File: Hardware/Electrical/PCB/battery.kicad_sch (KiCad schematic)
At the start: 33 parts, among them J2 jst, Q1 DMT6008LFG-7, Q2 DMT6008LFG-7, U6 BQ24600

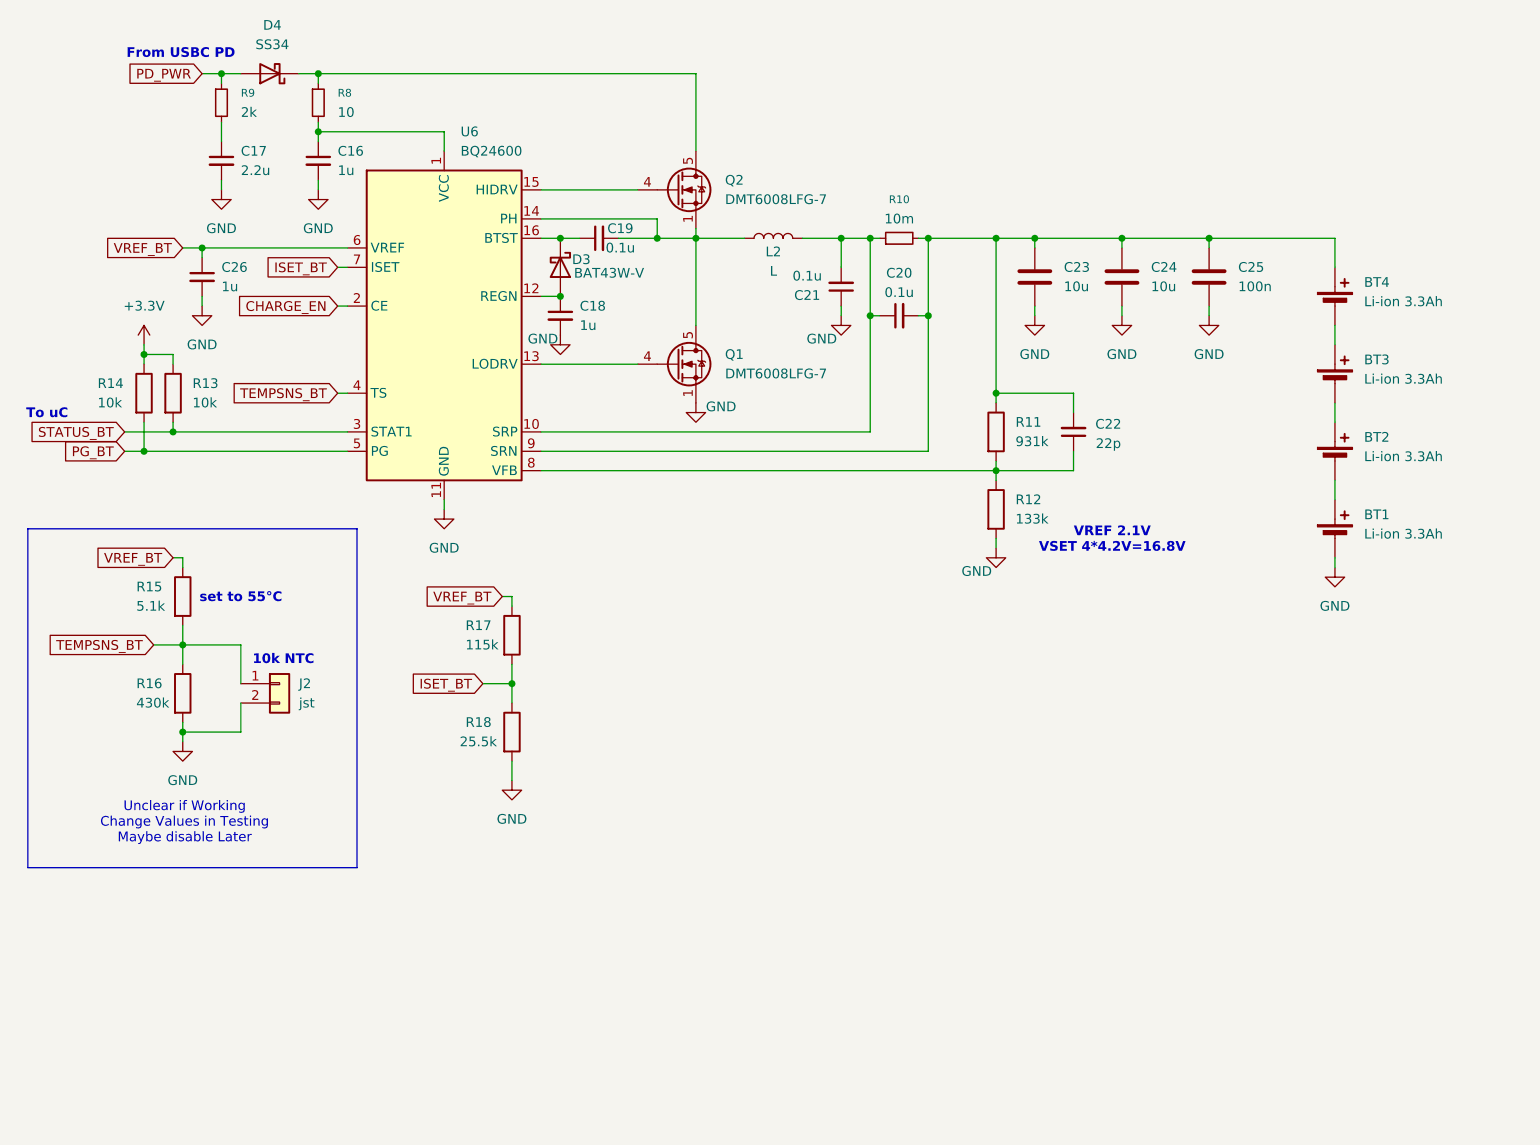
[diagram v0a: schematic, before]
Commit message: project state at start of school project
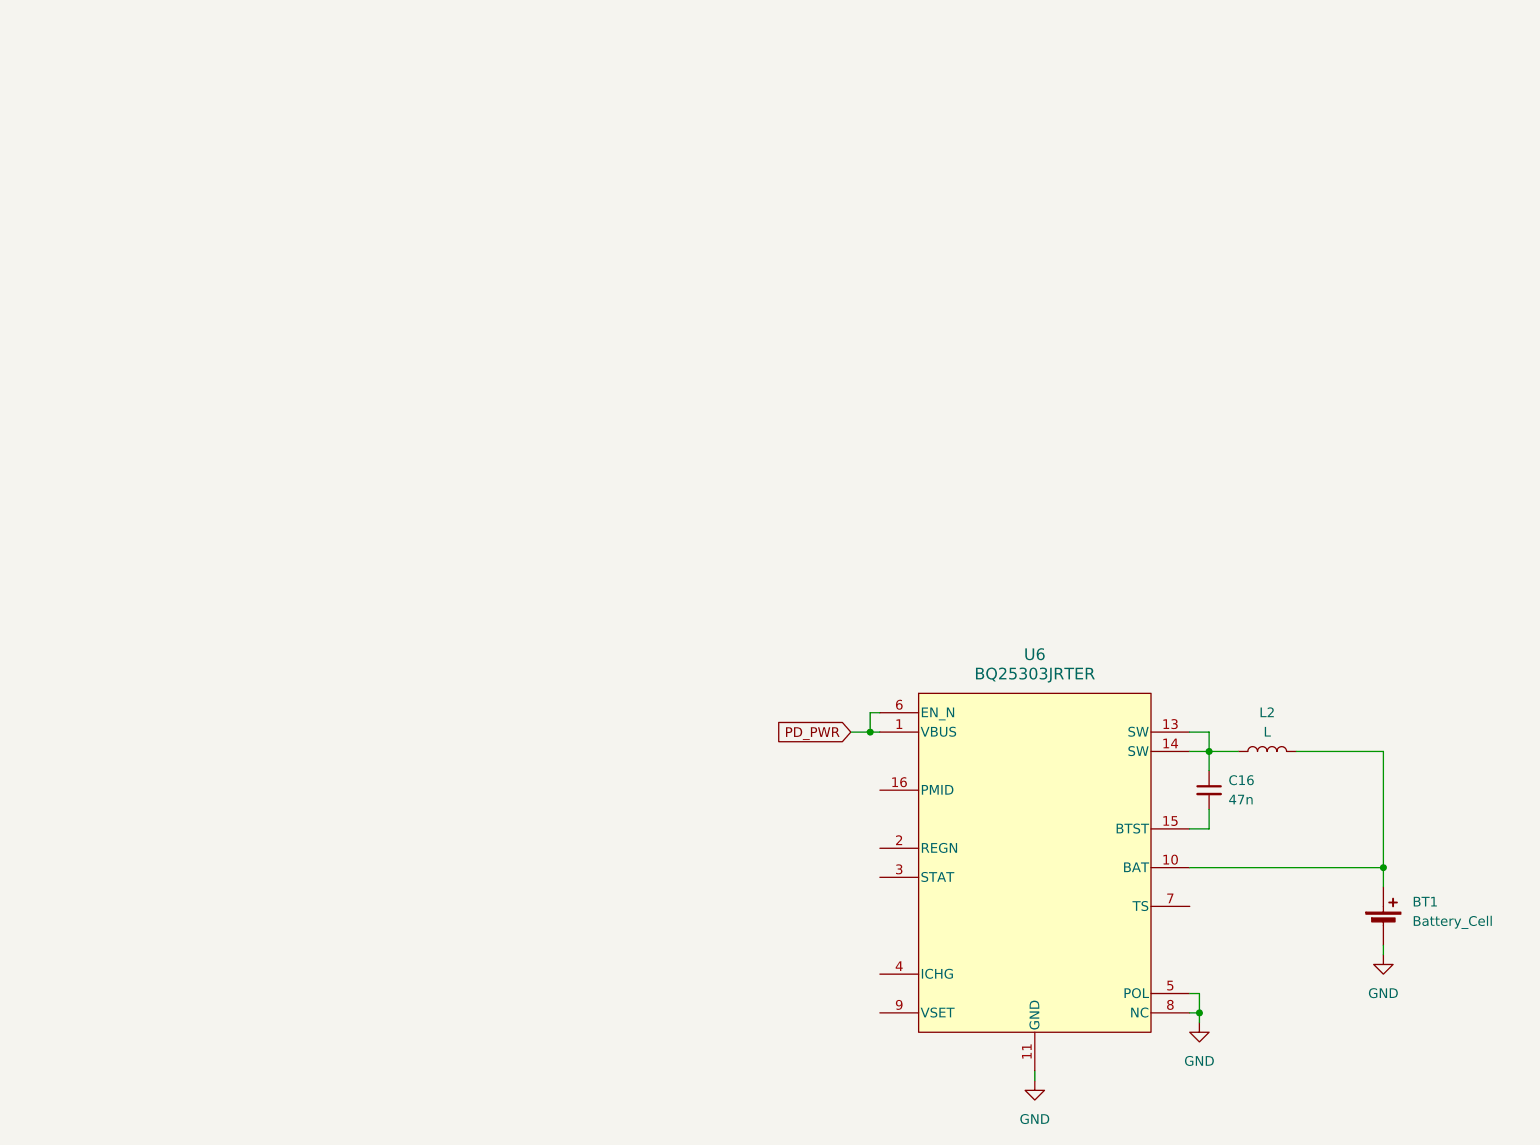
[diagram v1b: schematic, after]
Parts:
- removed BT2, BT3, BT4: Li-ion 3.3Ah, symbol Device:Battery_Cell
- removed C17: 2.2u, symbol Device:C_Small
- removed C18, C26: 1u, symbol Device:C_Small
- removed C19, C20, C21: 0.1u, symbol Device:C_Small
- removed C22: 22p, symbol Device:C_Small
- removed C23, C24: 10u, symbol Device:C
- removed C25: 100n, symbol Device:C
- removed D3: BAT43W-V, Diode_SMD:D_SOD-123, symbol Diode:BAT43W-V
- removed D4: SS34, Diode_SMD:D_SMC, symbol Diode:SS34
- removed J2: jst, symbol Connector_Generic:Conn_01x02
- removed Q1, Q2: DMT6008LFG-7, Package_SON:Diodes_PowerDI3333-8, symbol Transistor_FET:DMT6008LFG
- removed R10: 10m, symbol Device:R_Small
- removed R11: 931k, symbol Device:R
- removed R12: 133k, symbol Device:R
- removed R13, R14: 10k, symbol Device:R
- removed R15: 5.1k, symbol Device:R
- removed R16: 430k, symbol Device:R
- removed R17: 115k, symbol Device:R
- removed R18: 25.5k, symbol Device:R
- removed R8: 10, symbol Device:R_Small
- removed R9: 2k, symbol Device:R_Small
- removed U6: BQ24600, Package_DFN_QFN:Texas_RVA_VQFN-16-1EP_3.5x3.5mm_P0.5mm_EP2.14x2.14mm_ThermalVias, symbol Battery_Management:BQ24650
- added U6: BQ25303JRTER, RTE0016C, symbol BQ25303JRTER:BQ25303JRTER
- BT1: value Li-ion 3.3Ah -> Battery_Cell
- C16: value 1u -> 47n
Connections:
- net GND: now also U6.11 (GND), U6.12 (GND), U6.17 (PAD), U6.5 (POL), U6.8 (NC); no longer C16.2
- net PD_PWR: now also U6.1 (VBUS), U6.6 (EN_N)
- net at L2.1: now also C16.1, U6.13 (SW), U6.14 (SW)
- net at L2.2: now also BT1.1 (+), U6.10 (BAT)
- new net: C16.2, U6.15 (BTST)
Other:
- note removed: "10k NTC"
- note removed: "From USBC PD"
- note removed: "To uC"
- note removed: "Unclear if Working Change Values in Testing Maybe disable Later"
- note removed: "VREF 2.1V VSET 4*4.2V=16.8V"
- note removed: "set to 55°C"
